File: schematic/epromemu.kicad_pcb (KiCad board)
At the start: 2 copper layers, 82 x 54.1 mm, 18 parts, among them J1 EPROM Connector, U1 Teensy4.1, U2 74HC245, U3 74HC245, U4 74HC245, U5 74HC245, U6 74HC32

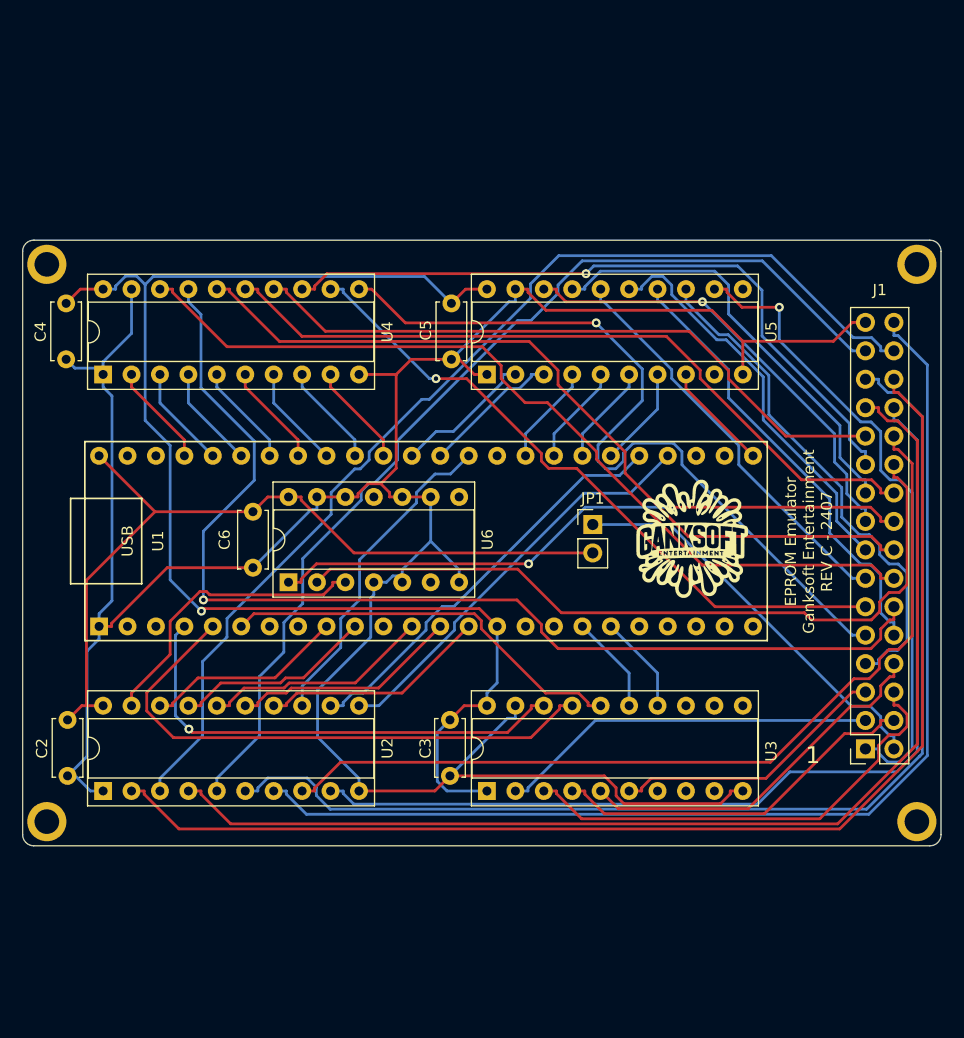
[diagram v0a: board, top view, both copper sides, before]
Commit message: Rev C schem/pcb
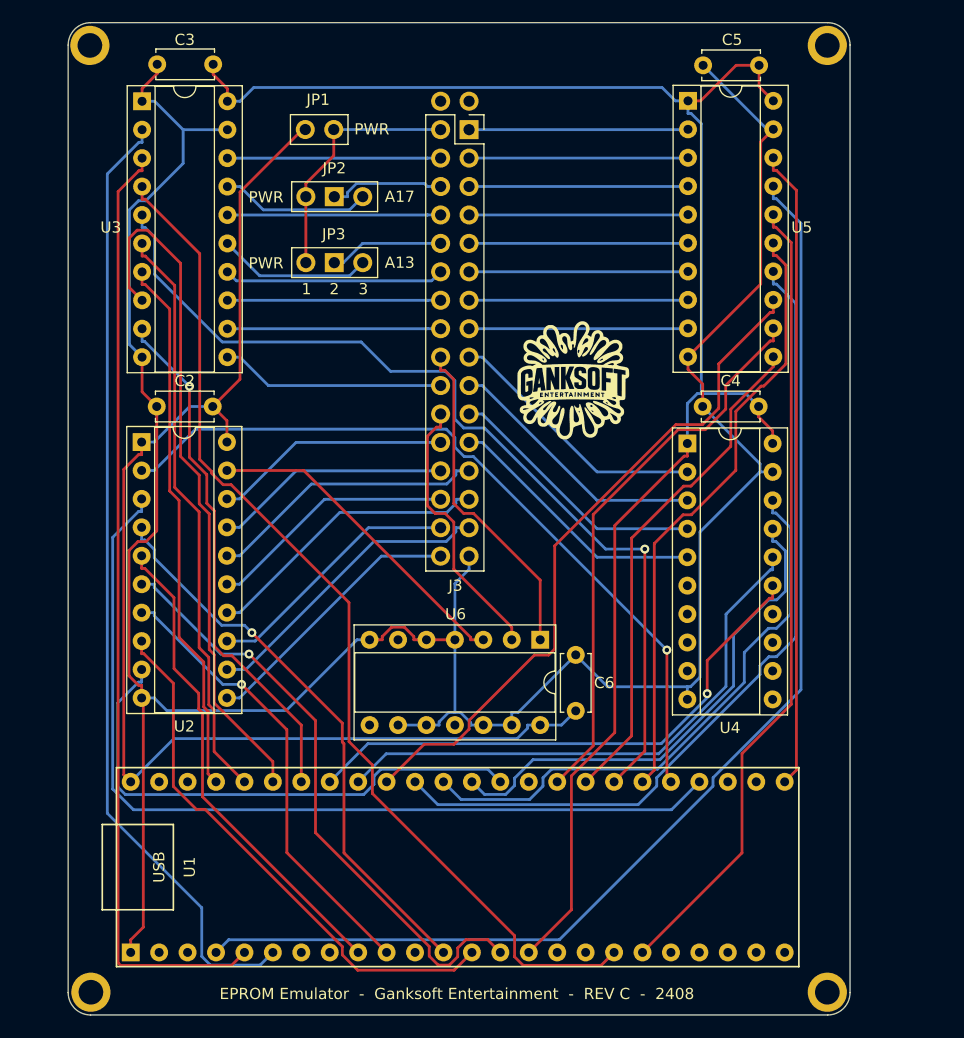
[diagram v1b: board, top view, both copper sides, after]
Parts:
- added JP2: A17, Connector_PinHeader_2.54mm:PinHeader_1x03_P2.54mm_Vertical, F.Cu at (130.7, 66.6)
- added JP3: A13, Connector_PinHeader_2.54mm:PinHeader_1x03_P2.54mm_Vertical, F.Cu at (130.7, 72.5)
- moved H4 75.3 mm to (111.5, 137.7)
- moved H3 71.4 mm to (177.3, 137.7)
- moved U3 68.9 mm to (116.1, 58.1), turned to 0 degrees
- moved J3 68.6 mm to (142.7, 60.6), turned to 0 degrees
- moved C4 62.5 mm to (171.2, 85.3), turned to 180 degrees
- moved C3 62.3 mm to (122.4, 54.8), turned to 180 degrees
- moved U4 52.6 mm to (164.8, 88.6), turned to 0 degrees
- moved JP1 42.2 mm to (133.2, 60.6), turned to -90 degrees
- moved C5 34.8 mm to (171.2, 54.9), turned to 180 degrees
- moved C6 33.9 mm to (154.8, 112.5), turned to 90 degrees
- moved U2 31.4 mm to (116.0, 88.5), turned to 0 degrees
- moved C2 30.9 mm to (122.4, 85.3), turned to 180 degrees
- moved U5 30.3 mm to (164.8, 58.0), turned to 0 degrees
- moved U1 29.3 mm to (144.3, 126.5)
- moved U6 23.1 mm to (151.6, 106.2), turned to -90 degrees
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- renumbered J1 to J3
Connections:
- net Net-(J1-Pin_32) renamed JP1_PWR
- J3 pad 28: A13_5V -> Net-(J3-Pin_28)
- J3 pad 30: A17_5V -> Net-(J3-Pin_30)
- U2 pad 1: GND -> +5V
- U2 pad 11: D6_3V3 -> D3_5V
- U2 pad 12: D7_3V3 -> D2_5V
- U2 pad 13: D3_3V3 -> D4_5V
- U2 pad 14: D1_3V3 -> D1_5V
- U2 pad 15: D2_3V3 -> D5_5V
- U2 pad 16: D0_3V3 -> D0_5V
- U2 pad 17: D4_3V3 -> D6_5V
- U2 pad 18: D5_3V3 -> D7_5V
- U2 pad 2: D5_5V -> D7_3V3
- U2 pad 3: D4_5V -> D6_3V3
- U2 pad 4: D0_5V -> D0_3V3
- U2 pad 5: D2_5V -> D5_3V3
- U2 pad 6: D1_5V -> D1_3V3
- U2 pad 7: D3_5V -> D4_3V3
- U2 pad 8: D7_5V -> D2_3V3
- U2 pad 9: D6_5V -> D3_3V3
- U3 pad 1: +3V3 -> GND
- U3 pad 11: unconnected-(U3-B7-Pad11) -> A10_5V
- U3 pad 12: unconnected-(U3-B6-Pad12) -> A11_5V
- U3 pad 13: unconnected-(U3-B5-Pad13) -> A9_5V
- U3 pad 14: A15_3V3 -> A8_5V
- U3 pad 15: A14_3V3 -> A13_5V
- U3 pad 16: A18_3V3 -> A14_5V
- U3 pad 17: A17_3V3 -> A17_5V
- U3 pad 18: A16_3V3 -> A18_5V
- U3 pad 2: A16_5V -> A18_3V3
- U3 pad 3: A17_5V -> A17_3V3
- U3 pad 4: A18_5V -> A14_3V3
- U3 pad 5: A14_5V -> A13_3V3
- U3 pad 6: A15_5V -> A8_3V3
- U3 pad 7: unconnected-(U3-A5-Pad7) -> A9_3V3
- U3 pad 8: unconnected-(U3-A6-Pad8) -> A11_3V3
- U3 pad 9: unconnected-(U3-A7-Pad9) -> A10_3V3
- U4 pad 1: GND -> +3V3
- U4 pad 11: A7_5V -> unconnected-(U4-B7-Pad11)
- U4 pad 12: A6_5V -> unconnected-(U4-B6-Pad12)
- U4 pad 13: A1_5V -> unconnected-(U4-B5-Pad13)
- U4 pad 14: A0_5V -> unconnected-(U4-B4-Pad14)
- U4 pad 15: A10_5V -> A0_3V3
- U4 pad 16: A11_5V -> A1_3V3
- U4 pad 17: A8_5V -> A2_3V3
- U4 pad 18: A9_5V -> A3_3V3
- U4 pad 2: A9_3V3 -> A3_5V
- U4 pad 3: A8_3V3 -> A2_5V
- U4 pad 4: A11_3V3 -> A1_5V
- U4 pad 5: A10_3V3 -> A0_5V
- U4 pad 6: A0_3V3 -> unconnected-(U4-A4-Pad6)
- U4 pad 7: A1_3V3 -> unconnected-(U4-A5-Pad7)
- U4 pad 8: A6_3V3 -> unconnected-(U4-A6-Pad8)
- U4 pad 9: A7_3V3 -> unconnected-(U4-A7-Pad9)
- U5 pad 1: GND -> +3V3
- U5 pad 11: unconnected-(U5-B7-Pad11) -> A4_3V3
- U5 pad 12: A19_5V -> A5_3V3
- U5 pad 13: A12_5V -> A6_3V3
- U5 pad 14: A13_5V -> A7_3V3
- U5 pad 15: A4_5V -> A12_3V3
- U5 pad 16: A5_5V -> A15_3V3
- U5 pad 17: A2_5V -> A16_3V3
- U5 pad 18: A3_5V -> A19_3V3
- U5 pad 2: A3_3V3 -> A19_5V
- U5 pad 3: A2_3V3 -> A16_5V
- U5 pad 4: A5_3V3 -> A15_5V
- U5 pad 5: A4_3V3 -> A12_5V
- U5 pad 6: A13_3V3 -> A7_5V
- U5 pad 7: A12_3V3 -> A6_5V
- U5 pad 8: A19_3V3 -> A5_5V
- U5 pad 9: unconnected-(U5-A7-Pad9) -> A4_5V
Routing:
- net D5_5V: track 109.3 -> 22.2 mm
- net A14_3V3: track 8.81 -> 92.9 mm
- net A8_5V: track 98.7 -> 19.7 mm, vias 1 -> 0
- net D0_5V: track 102.6 -> 25.0 mm
- net D3_5V: track 101.7 -> 24.3 mm
- net D1_5V: track 101.5 -> 26.0 mm
- net A13_3V3: track 8.99 -> 83.8 mm, vias 0 -> 1
- net D4_5V: track 96.9 -> 23.3 mm
- net A7_3V3: track 9.22 -> 75.6 mm
- net A16_3V3: track 43.0 -> 108.6 mm, vias 1 -> 0
- net D6_5V: track 86.8 -> 21.2 mm
- net A15_3V3: track 8.81 -> 72.2 mm
- net D2_5V: track 90.5 -> 27.1 mm
- net A9_5V: track 77.7 -> 19.1 mm
- net D7_5V: track 79.6 -> 21.2 mm
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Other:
- board size 82 x 54.1 mm -> 69.9 x 88.6 mm
- board text added: "2"
- board text added: "3"
- board text added: "EPROM Emulator - Ganksoft Entertainment - REV C - 2408"
- board text added: "PWR"
- board text removed: "EPROM Emulator Ganksoft Entertainment REV C - 2407"
